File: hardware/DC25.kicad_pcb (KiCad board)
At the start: 2 copper layers, 18 parts, among them P2 CONN_01X04, SW1 SW_DPDT_x2, U1 ATMEGA328P-AU, Y1 16MHz

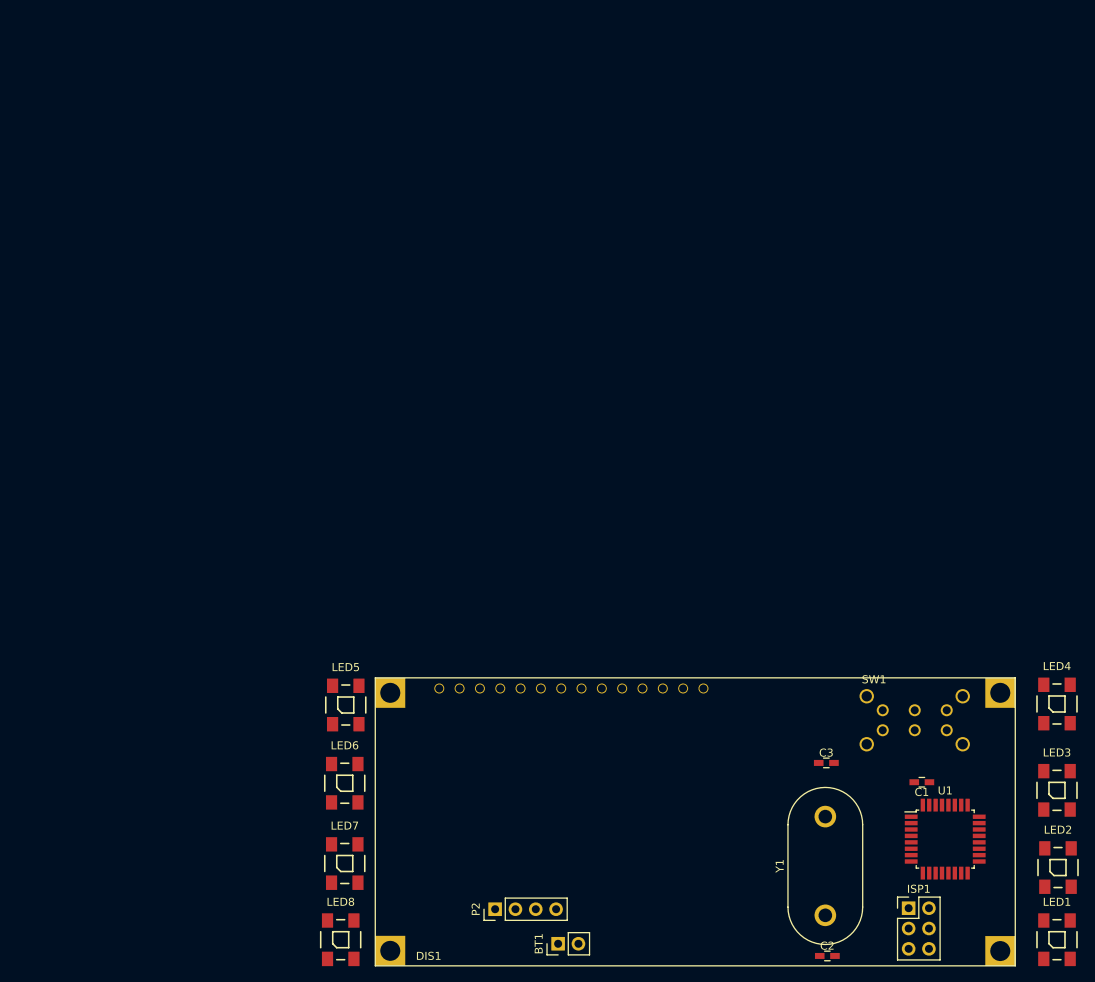
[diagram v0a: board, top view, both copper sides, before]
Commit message: Some progress
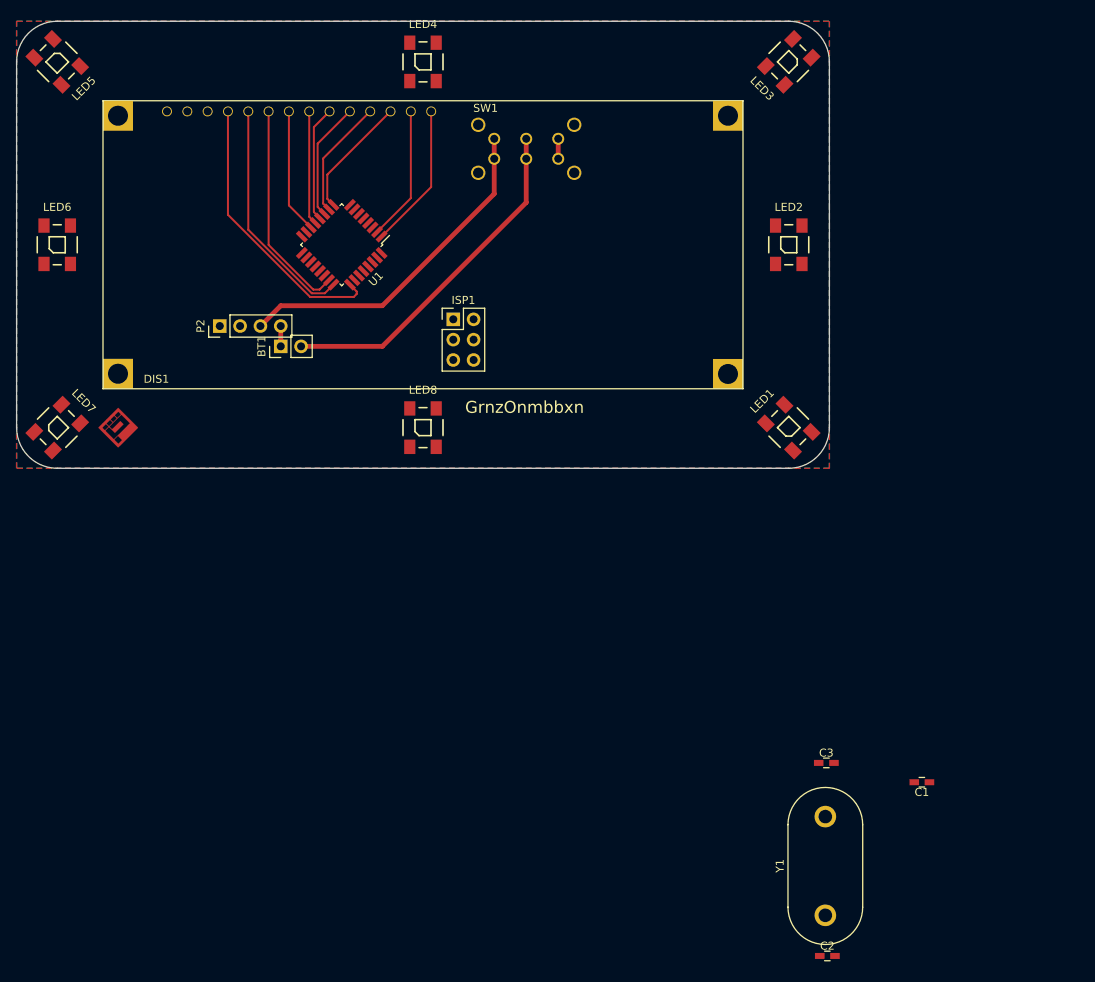
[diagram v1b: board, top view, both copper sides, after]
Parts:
- added G***: LOGO, images:p_logo_5_copper, F.Cu at (26.3, 64.6)
- added G***: LOGO, images:p_logo_5_mask, F.Cu at (26.3, 64.6)
- added G***: LOGO, footprints:bazooka_text, F.Cu at (41.4, 62.5)
- added G***: LOGO, footprints:bazooka, F.Cu at (56.3, 65.7)
- moved LED4 112.8 mm to (64.4, 18.9)
- moved U1 105.9 mm to (54.2, 41.8), turned to 225 degrees
- moved LED3 97.0 mm to (110.1, 18.9), turned to 135 degrees
- moved ISP1 93.1 mm to (68.2, 51.1)
- moved LED5 88.1 mm to (18.7, 18.9), turned to 225 degrees
- moved SW1 86.4 mm to (77.3, 29.8)
- moved LED2 84.8 mm to (110.1, 41.8)
- moved BT1 82.3 mm to (46.6, 54.5)
- moved P2 80.6 mm to (39.0, 51.9)
- moved DIS1 79.8 mm to (64.4, 41.8)
- moved LED6 76.3 mm to (18.7, 41.8)
- moved LED1 72.3 mm to (110.1, 64.6), turned to 45 degrees
- moved LED7 65.3 mm to (18.7, 64.6), turned to 315 degrees
- moved LED8 64.8 mm to (64.4, 64.6)
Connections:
- DIS1 pad 1: (no net) -> GND
- DIS1 pad 10: (no net) -> /DB3
- DIS1 pad 11: (no net) -> /DB4
- DIS1 pad 12: (no net) -> /DB5
- DIS1 pad 13: (no net) -> /DB6
- DIS1 pad 14: (no net) -> /DB7
- DIS1 pad 2: (no net) -> +5V
- DIS1 pad 3: (no net) -> Net-(DIS1-Pad3)
- DIS1 pad 4: (no net) -> /RS
- DIS1 pad 5: (no net) -> /RW
- DIS1 pad 6: (no net) -> /E
- DIS1 pad 7: (no net) -> /DB0
- DIS1 pad 8: (no net) -> /DB1
- DIS1 pad 9: (no net) -> /DB2
- U1 pad 1: /DB0 -> /DB7
- U1 pad 10: /DB3 -> /DB4
- U1 pad 11: /DB4 -> /DB3
- U1 pad 12: /DB5 -> /DB2
- U1 pad 13: /DB6 -> /DB1
- U1 pad 14: /DB7 -> /DB0
- U1 pad 2: /DB1 -> /DB6
- U1 pad 23: /RGB1 -> /E
- U1 pad 24: Net-(U1-Pad24) -> /RW
- U1 pad 25: Net-(U1-Pad25) -> /RS
- U1 pad 30: /RS -> /RGB1
- U1 pad 31: /RW -> Net-(U1-Pad31)
- U1 pad 32: /E -> Net-(U1-Pad32)
- U1 pad 9: /DB2 -> /DB5
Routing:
- net Net-(BT1-Pad2): track 0.00 -> 43.6 mm
- net GNDA: track 0.00 -> 43.0 mm
- net /RS: track 0.00 -> 34.9 mm
- net /RW: track 0.00 -> 29.2 mm
- net /E: track 0.00 -> 27.1 mm
- net /DB7: track 0.00 -> 18.2 mm
- net /DB6: track 0.00 -> 16.8 mm
- net /DB0: track 0.00 -> 15.7 mm
- net /DB5: track 0.00 -> 15.3 mm
- net /DB4: track 0.00 -> 15.0 mm
- net /DB3: track 0.00 -> 14.8 mm
- net /DB2: track 0.00 -> 14.5 mm
- net /DB1: track 0.00 -> 14.3 mm
- net +BATT: track 0.00 -> 2.54 mm
- net Net-(SW1-Pad3): track 0.00 -> 2.50 mm
- added copper zone on F.Cu, net +5V
- added copper zone on B.Cu, net GND
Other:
- board outline added: 101.6 x 55.9 mm
- board text added: "GrnzOnmbbxn"
